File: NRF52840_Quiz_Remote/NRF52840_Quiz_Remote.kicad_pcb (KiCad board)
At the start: 2 copper layers, 66 x 173 mm, 28 parts, among them J1 NRF_LEFT, J2 NRF_RIGHT, SW1 ANSWER_A, SW2 ANSWER_B, SW3 ANSWER_C, SW4 ANSWER_D, SW5 SUBMIT, SW6 POWER, SW7 RESET

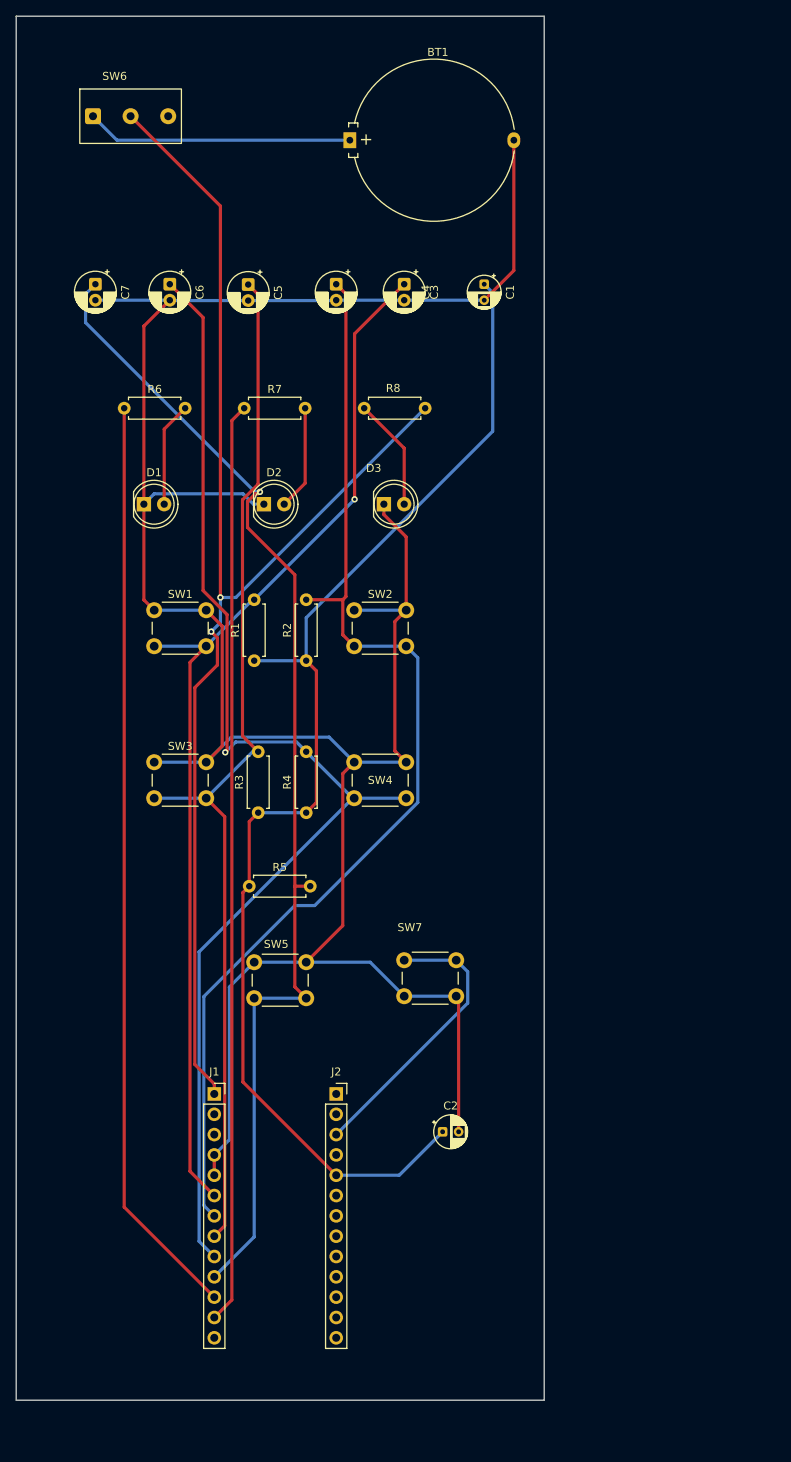
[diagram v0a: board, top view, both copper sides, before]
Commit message: PCB Final
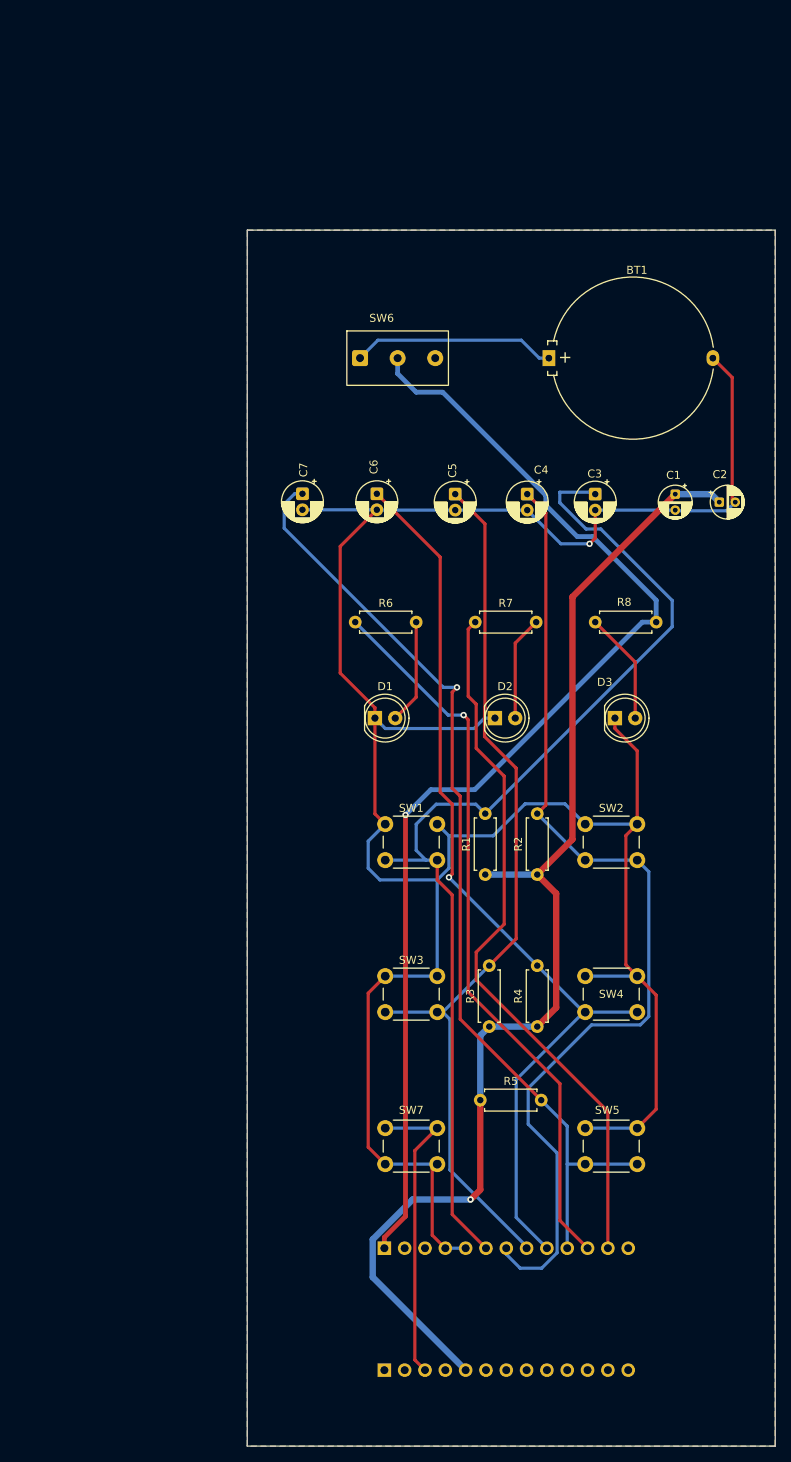
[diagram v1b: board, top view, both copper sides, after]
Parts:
- J1, J2: moved to B.Cu
- moved C2 86.0 mm to (129.4, 65.7)
- moved SW5 46.3 mm to (112.6, 144.0)
- moved SW6 45.0 mm to (89.2, 47.7)
- moved R5 39.4 mm to (99.5, 140.5)
- moved D2 39.4 mm to (101.3, 92.7)
- moved D3 39.4 mm to (116.3, 92.7)
- moved D1 39.4 mm to (86.3, 92.7)
- moved R3 39.4 mm to (100.6, 131.3)
- moved R4 39.4 mm to (106.6, 131.3)
- moved R1 39.4 mm to (100.1, 112.3)
- moved R2 39.4 mm to (106.6, 112.3)
- moved R6 39.4 mm to (83.9, 80.7)
- moved R7 39.4 mm to (98.9, 80.7)
- moved R8 39.4 mm to (113.9, 80.7)
- moved SW1 39.4 mm to (87.6, 106.0)
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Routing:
- net /BTN_D: track 153.7 -> 117.1 mm
- net /BTN_SUB: track 148.4 -> 120.7 mm
- net /LED_SENT: track 115.2 -> 88.8 mm
- net /LED_CONNECT: track 115.8 -> 91.4 mm, vias 0 -> 1
- net /BTN_C: track 132.2 -> 112.8 mm
- net /B+: track 165.2 -> 146.0 mm, vias 2 -> 1
- net /BTN_B: track 142.5 -> 125.9 mm
- net Net-(BT1-+): track 33.3 -> 25.5 mm
- net GND: track 329.5 -> 321.8 mm, vias 0 -> 1
- net /VCC: track 156.2 -> 152.1 mm, vias 0 -> 1
- net Net-(J2-Pin_3): track 35.7 -> 38.4 mm
- net /BTN_A: track 132.9 -> 134.0 mm, vias 1 -> 0
- added copper zone on B.Cu, net GND
- added copper zone on F.Cu, net GND
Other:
- board size 66 x 173 mm -> 66 x 152 mm
